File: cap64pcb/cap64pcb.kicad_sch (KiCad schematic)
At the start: 1 part

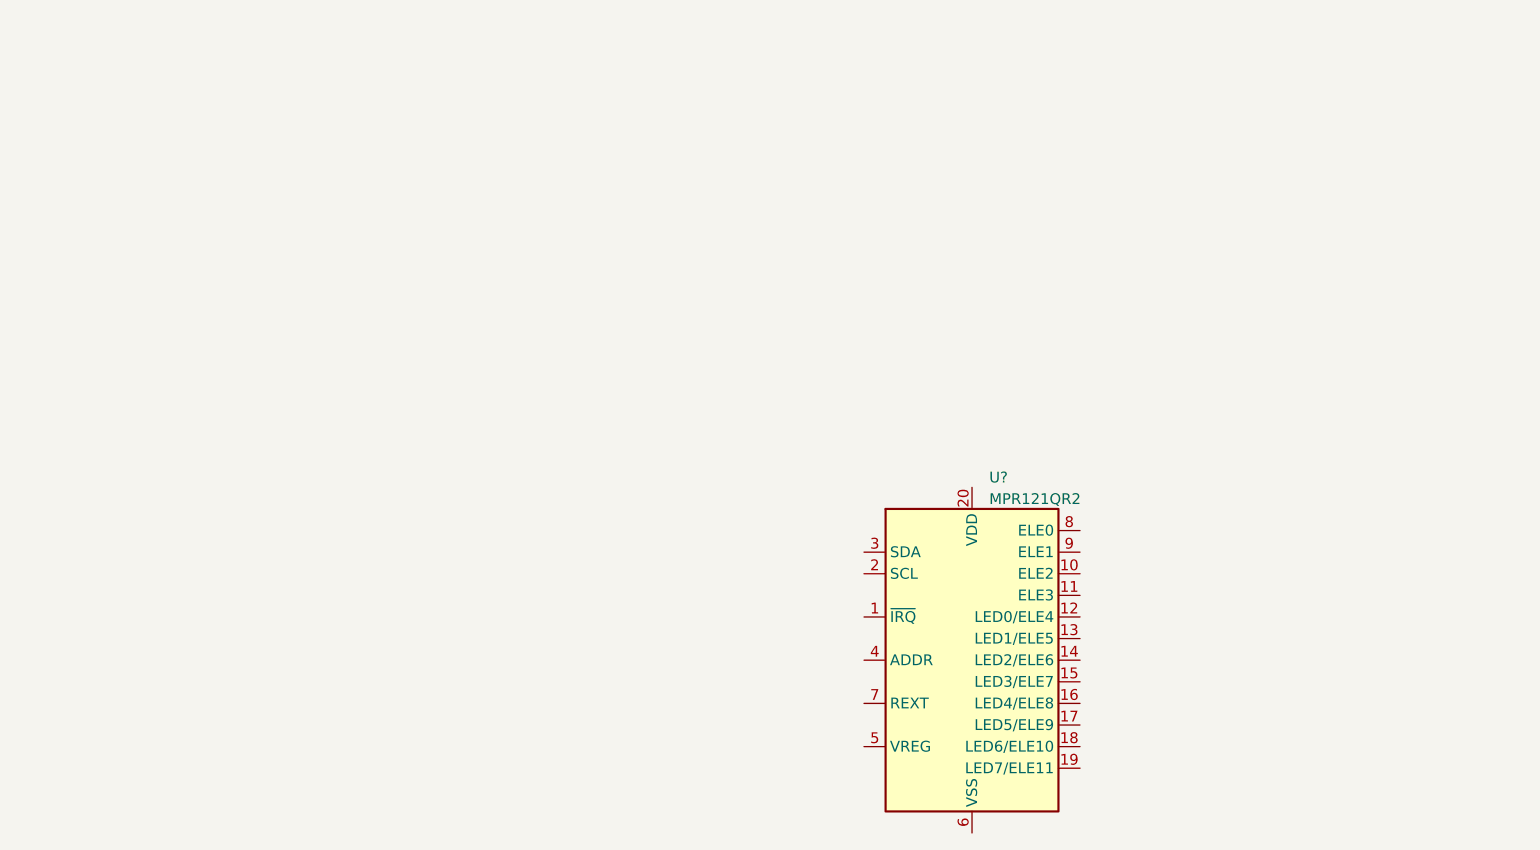
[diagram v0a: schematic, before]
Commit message: first draft sch
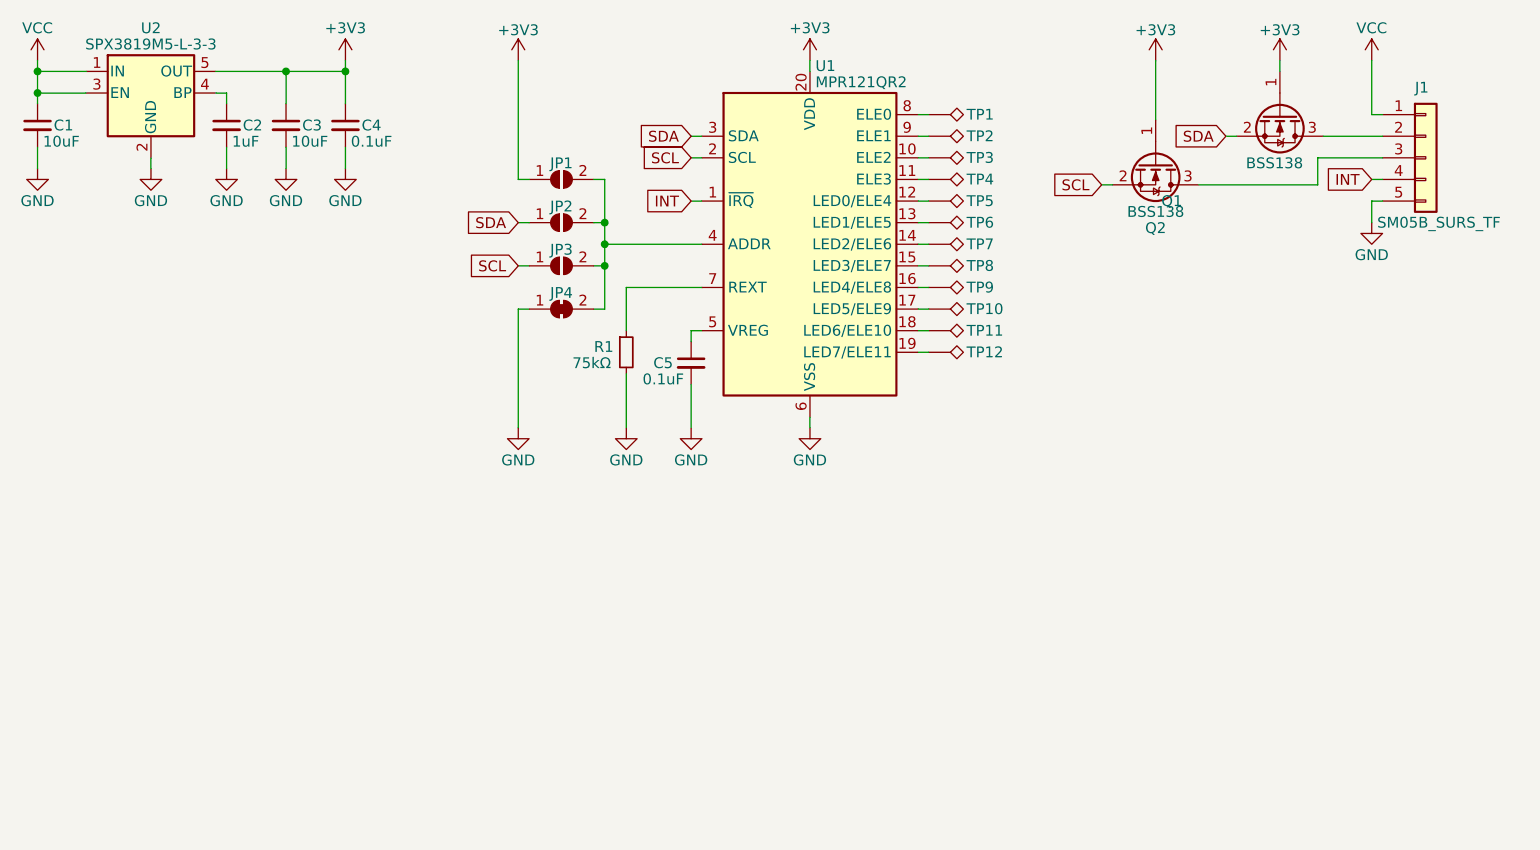
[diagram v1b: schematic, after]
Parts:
- added C1, C3: 10uF, Capacitor_SMD:C_0805_2012Metric, symbol Device:C_Small
- added C2: 1uF, Capacitor_SMD:C_0805_2012Metric, symbol Device:C_Small
- added C4, C5: 0.1uF, Capacitor_SMD:C_0805_2012Metric, symbol Device:C_Small
- added J1: SM05B_SURS_TF, Connector_JST:JST_SUR_SM05B-SURS-TF_1x05-1MP_P0.80mm_Horizontal, symbol Connector_Generic:Conn_01x05
- added JP1, JP2, JP3: SolderJumper_2_Open, Jumper:SolderJumper-2_P1.3mm_Open_RoundedPad1.0x1.5mm, symbol Jumper:SolderJumper_2_Open
- added JP4: SolderJumper_2_Bridged, Jumper:SolderJumper-2_P1.3mm_Bridged_RoundedPad1.0x1.5mm, symbol Jumper:SolderJumper_2_Bridged
- added Q1, Q2: BSS138, Package_TO_SOT_SMD:SOT-23, symbol Transistor_FET:BSS138
- added R1: 75kΩ, Resistor_SMD:R_0805_2012Metric, symbol Device:R_Small
- added TP1, TP10, TP11, TP12, TP2, TP3, TP4, TP5, TP6, TP7, TP8, TP9: TestPoint_Alt, symbol Connector:TestPoint_Alt
- added U2: SPX3819M5-L-3-3, Package_TO_SOT_SMD:SOT-23-5, symbol Regulator_Linear:SPX3819M5-L-3-3
- gave numbers to parts that had none: 1
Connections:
- net INT: now reaches U1.1 (~{IRQ})
- net INT: now also J1.4 (Pin_4)
- net at U1.10 (ELE2): now also TP3.1
- net at U1.11 (ELE3): now also TP4.1
- net at U1.12 (LED0/ELE4): now also TP5.1
- net at U1.13 (LED1/ELE5): now also TP6.1
- net at U1.14 (LED2/ELE6): now also TP7.1
- net at U1.15 (LED3/ELE7): now also TP8.1
- net at U1.16 (LED4/ELE8): now also TP9.1
- net at U1.17 (LED5/ELE9): now also TP10.1
- net at U1.18 (LED6/ELE10): now also TP11.1
- net at U1.19 (LED7/ELE11): now also TP12.1
- net SCL: now reaches U1.2 (SCL)
- net SCL: now also JP3.1 (A), Q2.2 (S)
- net +3V3: now reaches U1.20 (VDD)
- net +3V3: now also C3.1, C4.1, JP1.1 (A), Q1.1 (G), Q2.1 (G), U2.5 (OUT)
- net SDA: now reaches U1.3 (SDA)
- net SDA: now also JP2.1 (A), Q1.2 (S)
- net at U1.4 (ADDR): now also JP1.2 (B), JP2.2 (B), JP3.2 (B), JP4.2 (B)
- net at U1.5 (VREG): now also C5.1
- net GND: now reaches U1.6 (VSS)
- net GND: now also C1.2, C2.2, C3.2, C4.2, C5.2, J1.5 (Pin_5), JP4.1 (A), R1.2, U2.2 (GND)
- net at U1.7 (REXT): now also R1.1
- net at U1.8 (ELE0): now also TP1.1
- net at U1.9 (ELE1): now also TP2.1
- new net: C2.1, U2.4 (BP)
- new net: J1.2 (Pin_2), Q1.3 (D)
- new net: J1.3 (Pin_3), Q2.3 (D)
- new net VCC: C1.1, J1.1 (Pin_1), U2.1 (IN), U2.3 (EN)
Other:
- company: (none) -> beadybiddle
- title: (none) -> cap64
- moved on the sheet: U1
